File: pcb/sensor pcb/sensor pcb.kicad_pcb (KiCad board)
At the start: 2 copper layers, 26.5 x 16 mm, 1 part

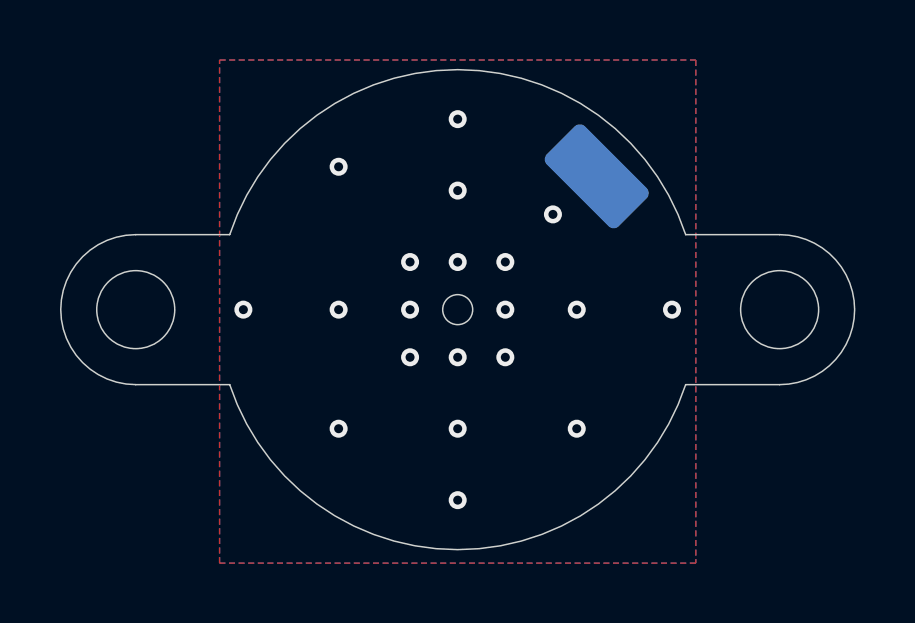
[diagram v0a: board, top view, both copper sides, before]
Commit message: bidibou
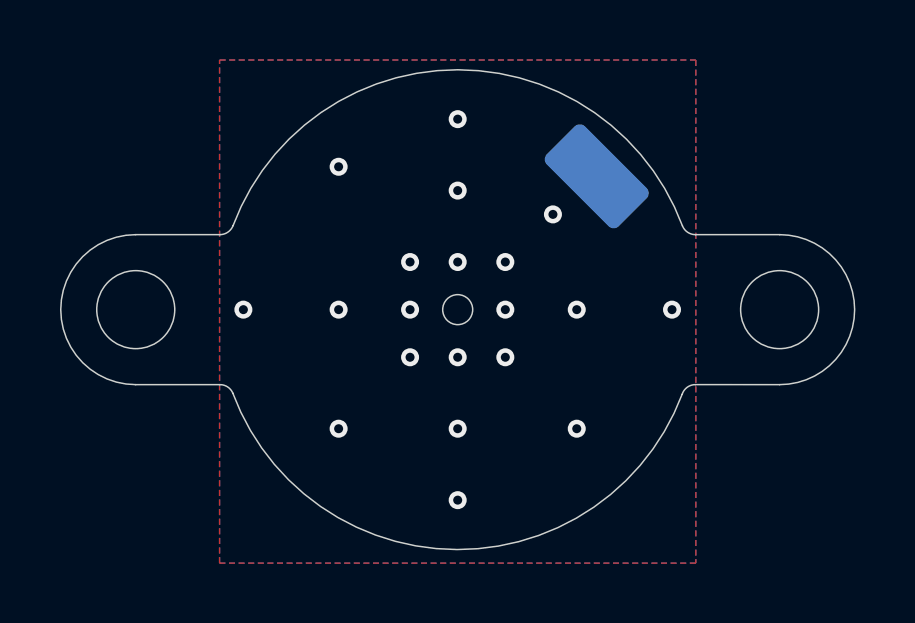
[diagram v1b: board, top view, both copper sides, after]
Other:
- outline, holes or cut-outs redrawn
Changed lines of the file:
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@@
 	)
 	(gr_arc
-		(start 159.088158 92.75)
-		(mid 166.6875 87.25)
-		(end 174.286842 92.75)
+		(start 159.199999 92.449076)
+		(mid 166.693769 87.253993)
+		(end 174.18 92.459935)
+		(stroke
+			(width 0.05)
+			(type default)
+		)
+		(layer "Edge.Cuts")
+	)
+	(gr_arc
+		(start 158.76 97.75)
+		(mid 159.017364 97.824941)
+		(end 159.19 98.03)
 		(stroke
 			(width 0.05)
@@
 	)
 	(gr_arc
-		(start 174.286842 97.75)
-		(mid 166.6875 103.25)
-		(end 159.088158 97.75)
+		(start 174.17 98.070003)
+		(mid 166.666098 103.247106)
+		(end 159.19 98.029932)
+		(stroke
+			(width 0.05)
+			(type default)
+		)
+		(layer "Edge.Cuts")
+	)
+	(gr_arc
+		(start 159.2 92.449076)
+		(mid 159.026383 92.667357)
+		(end 158.76 92.75)
 		(stroke
 			(width 0.05)
@@
 	)
 	(gr_line
-		(start 159.088159 92.75)
+		(start 158.76 92.75)
 		(end 155.956 92.75)
 		(stroke
@@
 	)
 	(gr_line
-		(start 174.286841 97.75)
+		(start 174.61 97.749102)
 		(end 177.419 97.75)
 		(stroke
@@
 	)
 	(gr_line
-		(start 174.286842 92.75)
+		(start 174.616304 92.75)
 		(end 177.419 92.75)
 		(stroke
@@
 	)
 	(gr_line
-		(start 159.088158 97.749997)
+		(start 158.76 97.750001)
 		(end 155.956 97.75)
+		(stroke
+			(width 0.05)
+			(type default)
+		)
+		(layer "Edge.Cuts")
+	)
+	(gr_arc
+		(start 174.17 98.07)
+		(mid 174.337858 97.838049)
+		(end 174.61 97.749076)
+		(stroke
+			(width 0.05)
+			(type default)
+		)
+		(layer "Edge.Cuts")
+	)
+	(gr_arc
+		(start 174.616383 92.75)
+		(mid 174.353897 92.671653)
+		(end 174.18 92.46)
 		(stroke
 			(width 0.05)
@@
 		(end 174.6875 95.25)
 		(stroke
-			(width 0.1)
+			(width 0.01)
 			(type solid)
 		)
